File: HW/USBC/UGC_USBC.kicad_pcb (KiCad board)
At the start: 2 copper layers, 30 x 12 mm, 3 parts, among them J1 UJ31-CH-G1-SMT-TR

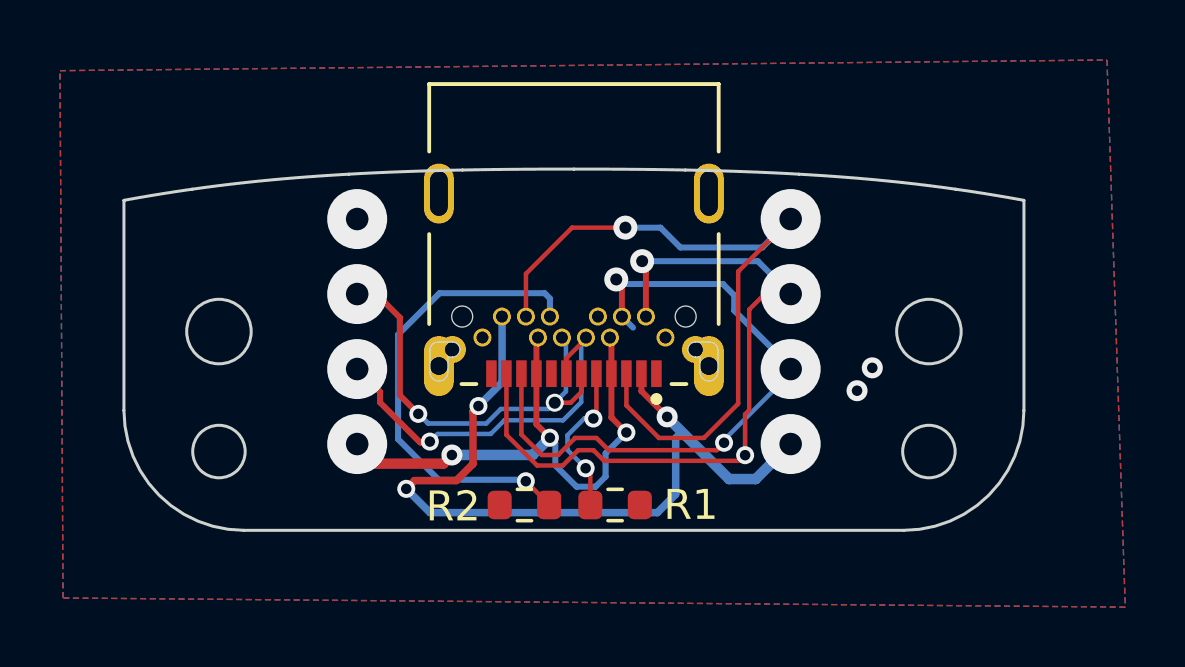
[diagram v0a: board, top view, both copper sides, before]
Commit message: Production files
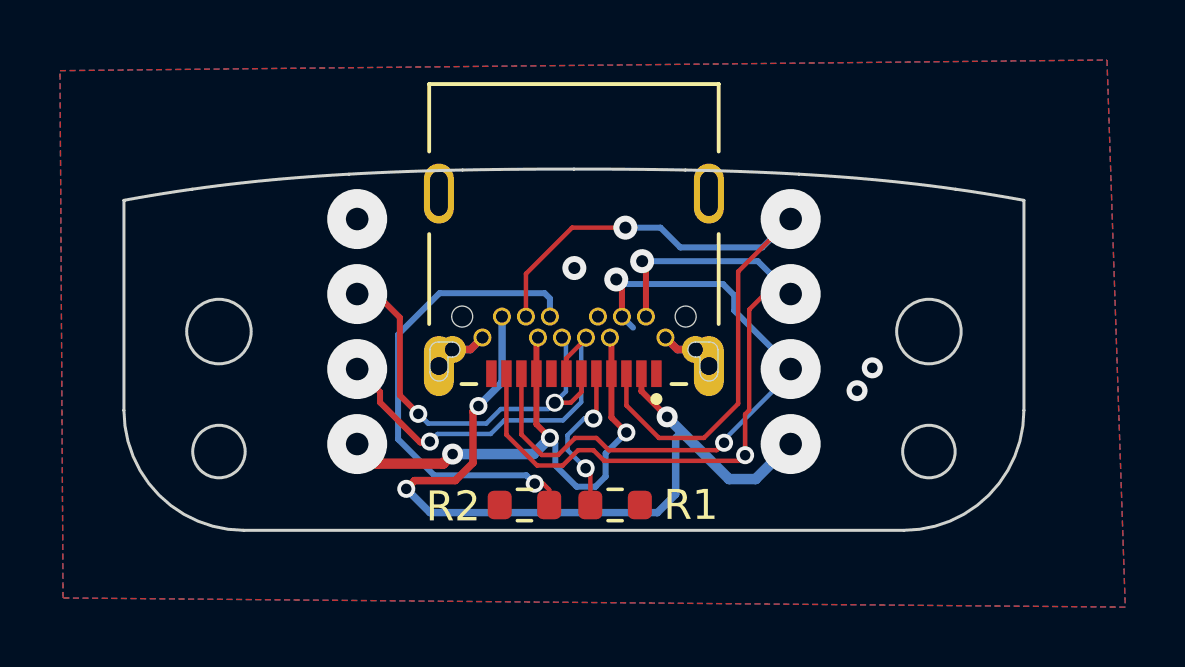
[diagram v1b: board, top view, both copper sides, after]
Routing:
- net GND: track 0.08 -> 4.74 mm, vias 3 -> 4
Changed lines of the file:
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@@
   (gr_curve (pts (xy 232.627911 147.228253) (xy 231.395241 147.204331) (xy 230.150122 147.197125) (xy 228.9162 147.197125))
     (stroke (width 0.1) (type solid)) (layer "Edge.Cuts"))
+  (segment (start 225.466178 153.2124) (end 225.866178 152.8124) (width 0.25) (layer "F.Cu") (net 1))
+  (segment (start 224.866178 153.2124) (end 225.466178 153.2124) (width 0.25) (layer "F.Cu") (net 1))
+  (segment (start 232.966178 153.2124) (end 232.366178 153.2124) (width 0.25) (layer "F.Cu") (net 1))
   (segment (start 231.0384 158.3944) (end 231.1136 158.3944) (width 0.25) (layer "F.Cu") (net 1))
+  (segment (start 232.366178 153.2124) (end 231.966178 152.8124) (width 0.25) (layer "F.Cu") (net 1))
   (via (at 238.8616 153.8224) (size 0.7) (drill 0.35) (layers "F.Cu" "B.Cu") (free) (net 1))
+  (via (at 228.9302 150.495) (size 0.8) (drill 0.4) (layers "F.Cu" "B.Cu") (free) (net 1))
   (via (at 238.3536 154.5844) (size 0.7) (drill 0.35) (layers "F.Cu" "B.Cu") (free) (net 1))
   (via (at 221.6912 148.8624) (size 2) (drill 0.75) (layers "F.Cu" "B.Cu") (net 1))
-  (segment (start 223.600929 157.5816) (end 224.9932 157.5816) (width 0.25) (layer "F.Cu") (net 2))
+  (segment (start 232.366178 153.2124) (end 231.966178 152.8124) (width 0.25) (layer "B.Cu") (net 1))
+  (segment (start 224.866178 153.2124) (end 225.466178 153.2124) (width 0.25) (layer "B.Cu") (net 1))
+  (segment (start 232.966178 153.2124) (end 232.366178 153.2124) (width 0.25) (layer "B.Cu") (net 1))
+  (segment (start 225.466178 153.2124) (end 225.866178 152.8124) (width 0.25) (layer "B.Cu") (net 1))
+  (segment (start 223.326942 157.855587) (end 223.600929 157.5816) (width 0.25) (layer "F.Cu") (net 2))
   (segment (start 232.022829 155.456574) (end 231.166178 154.599923) (width 0.2) (layer "F.Cu") (net 2))
+  (segment (start 223.600929 157.5816) (end 224.960628 157.5816) (width 0.25) (layer "F.Cu") (net 2))
   (segment (start 231.166178 154.599923) (end 231.166178 154.0174) (width 0.2) (layer "F.Cu") (net 2))
-  (segment (start 223.326942 157.855587) (end 223.600929 157.5816) (width 0.25) (layer "F.Cu") (net 2))
-  (segment (start 224.9932 157.5816) (end 225.552 157.0228) (width 0.25) (layer "F.Cu") (net 2))
-  (segment (start 225.552 157.0228) (end 225.552 155.27582) (width 0.25) (layer "F.Cu") (net 2))
   (segment (start 225.552 155.27582) (end 225.73306 155.09476) (width 0.25) (layer "F.Cu") (net 2))
+  (segment (start 224.960628 157.5816) (end 225.552 156.990228) (width 0.25) (layer "F.Cu") (net 2))
+  (segment (start 225.552 156.990228) (end 225.552 155.27582) (width 0.25) (layer "F.Cu") (net 2))
   (via (at 232.022829 155.456574) (size 0.7) (drill 0.35) (layers "F.Cu" "B.Cu") (net 2))
   (via (at 236.1412 156.3624) (size 2) (drill 0.75) (layers "F.Cu" "B.Cu") (net 2))
@@
   (segment (start 231.8004 149.1488) (end 232.4608 149.8092) (width 0.2) (layer "B.Cu") (net 3))
   (segment (start 228.115158 156.151348) (end 227.666178 155.702368) (width 0.2) (layer "F.Cu") (net 4))
-  (segment (start 224.848896 156.727373) (end 224.561164 157.015105) (width 0.35) (layer "F.Cu") (net 4))
   (segment (start 227.666178 155.702368) (end 227.666178 154.0174) (width 0.2) (layer "F.Cu") (net 4))
+  (segment (start 222.343905 157.015105) (end 221.6912 156.3624) (width 0.35) (layer "F.Cu") (net 4))
   (segment (start 230.664205 155.976669) (end 230.166178 155.478642) (width 0.2) (layer "F.Cu") (net 4))
   (segment (start 227.666178 152.8624) (end 227.666178 154.0174) (width 0.2) (layer "F.Cu") (net 4))
   (segment (start 230.166178 152.8624) (end 230.166178 154.0174) (width 0.2) (layer "F.Cu") (net 4))
+  (segment (start 224.554868 157.015105) (end 222.343905 157.015105) (width 0.35) (layer "F.Cu") (net 4))
   (segment (start 227.716178 152.8124) (end 227.666178 152.8624) (width 0.2) (layer "F.Cu") (net 4))
+  (segment (start 224.873189 156.696784) (end 224.554868 157.015105) (width 0.35) (layer "F.Cu") (net 4))
   (segment (start 230.116178 152.8124) (end 230.166178 152.8624) (width 0.2) (layer "F.Cu") (net 4))
-  (segment (start 224.561164 157.015105) (end 222.343905 157.015105) (width 0.35) (layer "F.Cu") (net 4))
   (segment (start 230.166178 155.478642) (end 230.166178 154.0174) (width 0.2) (layer "F.Cu") (net 4))
-  (segment (start 222.343905 157.015105) (end 221.6912 156.3624) (width 0.35) (layer "F.Cu") (net 4))
   (via (at 228.115158 156.151348) (size 0.6) (drill 0.35) (layers "F.Cu" "B.Cu") (net 4))
   (via (at 230.664205 155.976669) (size 0.6) (drill 0.35) (layers "F.Cu" "B.Cu") (net 4))
   (via (at 221.6912 156.3624) (size 2) (drill 0.75) (layers "F.Cu" "B.Cu") (net 4))
-  (via (at 224.848896 156.727373) (size 0.7) (drill 0.35) (layers "F.Cu" "B.Cu") (net 4))
+  (via (at 224.873189 156.696784) (size 0.7) (drill 0.35) (layers "F.Cu" "B.Cu") (net 4))
   (segment (start 228.2952 156.33139) (end 228.2952 157.0736) (width 0.2) (layer "B.Cu") (net 4))
-  (segment (start 227.539133 156.727373) (end 228.115158 156.151348) (width 0.35) (layer "B.Cu") (net 4))
   (segment (start 229.634595 157.7848) (end 229.9716 157.447795) (width 0.2) (layer "B.Cu") (net 4))
   (segment (start 229.9716 156.669274) (end 230.664205 155.976669) (width 0.2) (layer "B.Cu") (net 4))
-  (segment (start 224.848896 156.727373) (end 227.539133 156.727373) (width 0.35) (layer "B.Cu") (net 4))
+  (segment (start 227.569722 156.696784) (end 228.115158 156.151348) (width 0.35) (layer "B.Cu") (net 4))
   (segment (start 229.0064 157.7848) (end 229.634595 157.7848) (width 0.2) (layer "B.Cu") (net 4))
   (segment (start 228.2952 157.0736) (end 229.0064 157.7848) (width 0.2) (layer "B.Cu") (net 4))
   (segment (start 228.115158 156.151348) (end 228.2952 156.33139) (width 0.2) (layer "B.Cu") (net 4))
+  (segment (start 224.873189 156.696784) (end 227.569722 156.696784) (width 0.35) (layer "B.Cu") (net 4))
   (segment (start 229.9716 157.447795) (end 229.9716 156.669274) (width 0.2) (layer "B.Cu") (net 4))
   (segment (start 229.307073 157.168869) (end 229.4636 157.325396) (width 0.15) (layer "F.Cu") (net 5))
@@
   (segment (start 231.1908 150.2664) (end 235.0452 150.2664) (width 0.2) (layer "B.Cu") (net 10))
   (segment (start 235.0452 150.2664) (end 236.1412 151.3624) (width 0.2) (layer "B.Cu") (net 10))
-  (segment (start 228.092 158.381734) (end 228.092 158.3944) (width 0.15) (layer "F.Cu") (net 11))
-  (segment (start 227.312372 157.602106) (end 228.092 158.381734) (width 0.15) (layer "F.Cu") (net 11))
-  (via (at 227.312372 157.602106) (size 0.6) (drill 0.35) (layers "F.Cu" "B.Cu") (net 11))
+  (segment (start 228.092 157.8864) (end 228.092 158.3944) (width 0.15) (layer "F.Cu") (net 11))
+  (segment (start 227.6094 157.6832) (end 227.8888 157.6832) (width 0.15) (layer "F.Cu") (net 11))
+  (segment (start 227.8888 157.6832) (end 228.092 157.8864) (width 0.15) (layer "F.Cu") (net 11))
+  (via (at 227.6094 157.6832) (size 0.6) (drill 0.35) (layers "F.Cu" "B.Cu") (net 11))
   (segment (start 227.9396 151.3332) (end 228.116178 151.509778) (width 0.2) (layer "B.Cu") (net 11))
-  (segment (start 224.404427 157.551627) (end 223.054353 156.201553) (width 0.2) (layer "B.Cu") (net 11))
   (segment (start 223.054353 156.201553) (end 223.054353 152.713247) (width 0.2) (layer "B.Cu") (net 11))
   (segment (start 228.116178 151.509778) (end 228.116178 152.1124) (width 0.2) (layer "B.Cu") (net 11))
-  (segment (start 227.261893 157.551627) (end 224.404427 157.551627) (width 0.2) (layer "B.Cu") (net 11))
   (segment (start 223.054353 152.713247) (end 224.4344 151.3332) (width 0.2) (layer "B.Cu") (net 11))
+  (segment (start 224.2566 157.4038) (end 223.054353 156.201553) (width 0.2) (layer "B.Cu") (net 11))
+  (segment (start 227.6094 157.6832) (end 227.33 157.4038) (width 0.2) (layer "B.Cu") (net 11))
+  (segment (start 227.33 157.4038) (end 224.2566 157.4038) (width 0.2) (layer "B.Cu") (net 11))
   (segment (start 224.4344 151.3332) (end 227.9396 151.3332) (width 0.2) (layer "B.Cu") (net 11))
-  (segment (start 227.312372 157.602106) (end 227.261893 157.551627) (width 0.2) (layer "B.Cu") (net 11))
   (zone (net 1) (net_name "GND") (layers "F&B.Cu") (hatch edge 0.5)
     (connect_pads (clearance 0.2))
